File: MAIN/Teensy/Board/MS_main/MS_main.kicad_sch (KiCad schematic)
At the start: 32 parts, among them J1 External 5V, J10 RM_Motor, J11 RM_Motor, J12 Capacitive Soil Moisture Sens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, J14 LED, J15 LED_U, J16 RM_Motor, J17 RM_Motor, J18 RM_Motor, J19 RM_Motor, J2 BLD-510B_1, J20 RM_Motor, J21 Teensy4.1_Extention, J22 AE-PCA9685_Extention, J23 AE-PCA9685_Remaining, J3 BLD-510B_2, J4 BLD-510B_3, J5 BLD-510B_4, J6 BLD-510B_5, J7 SG_90-HV, J8 RM_Motor, J9 RM_Motor, U1 Teensy4.1

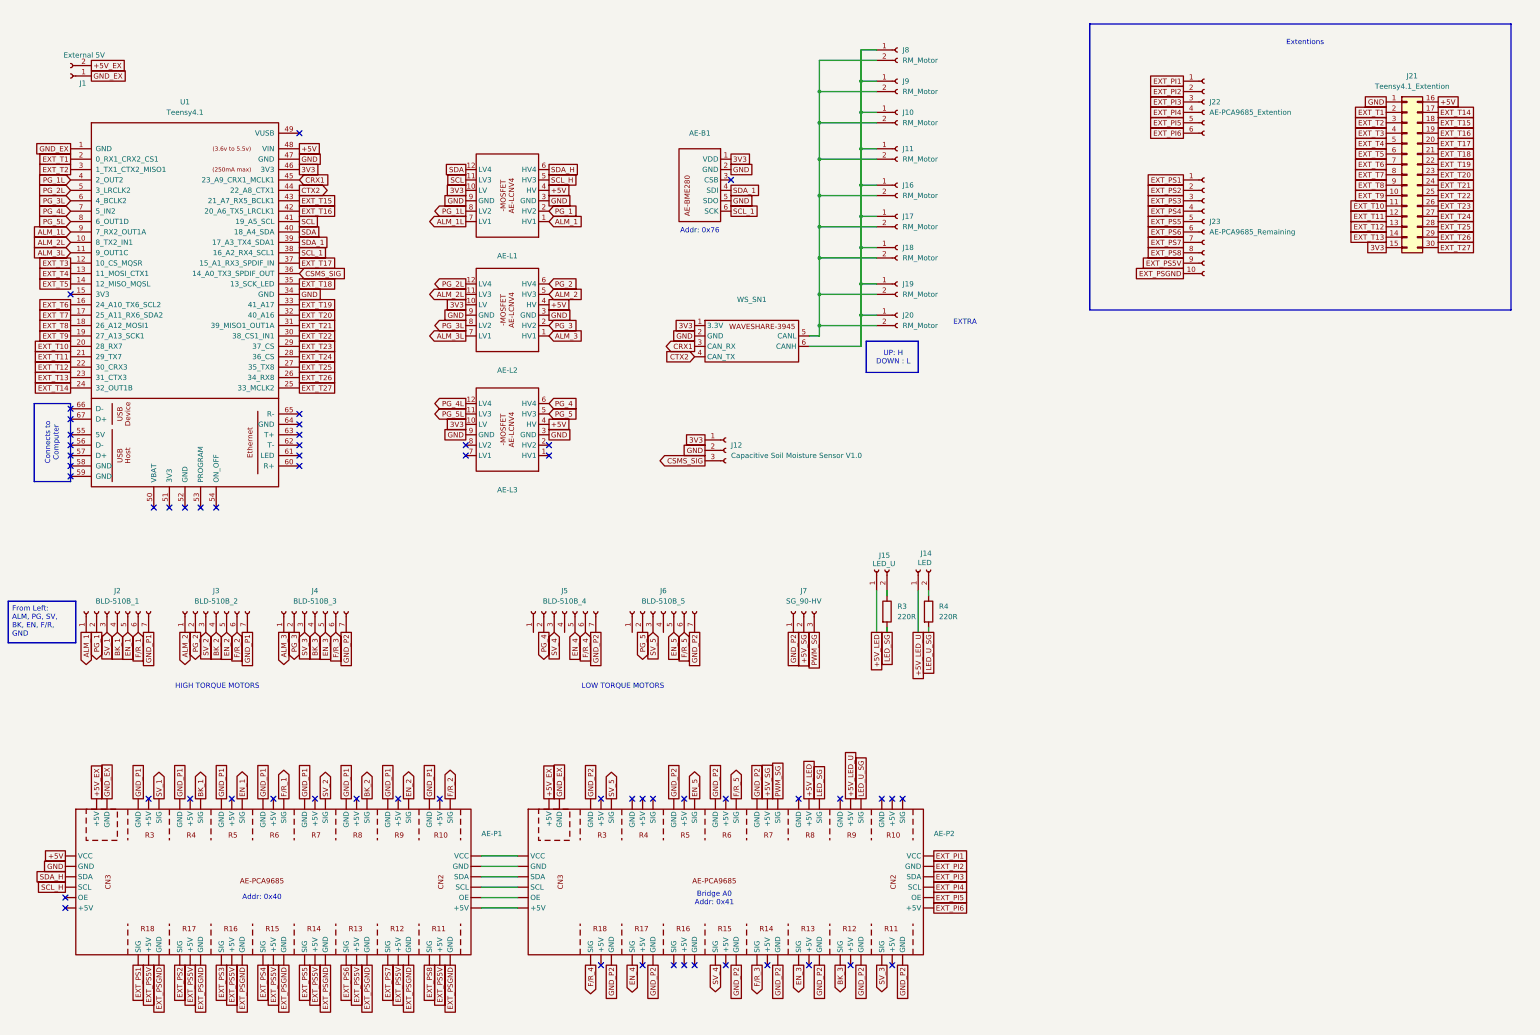
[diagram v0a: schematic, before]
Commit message: board revamp
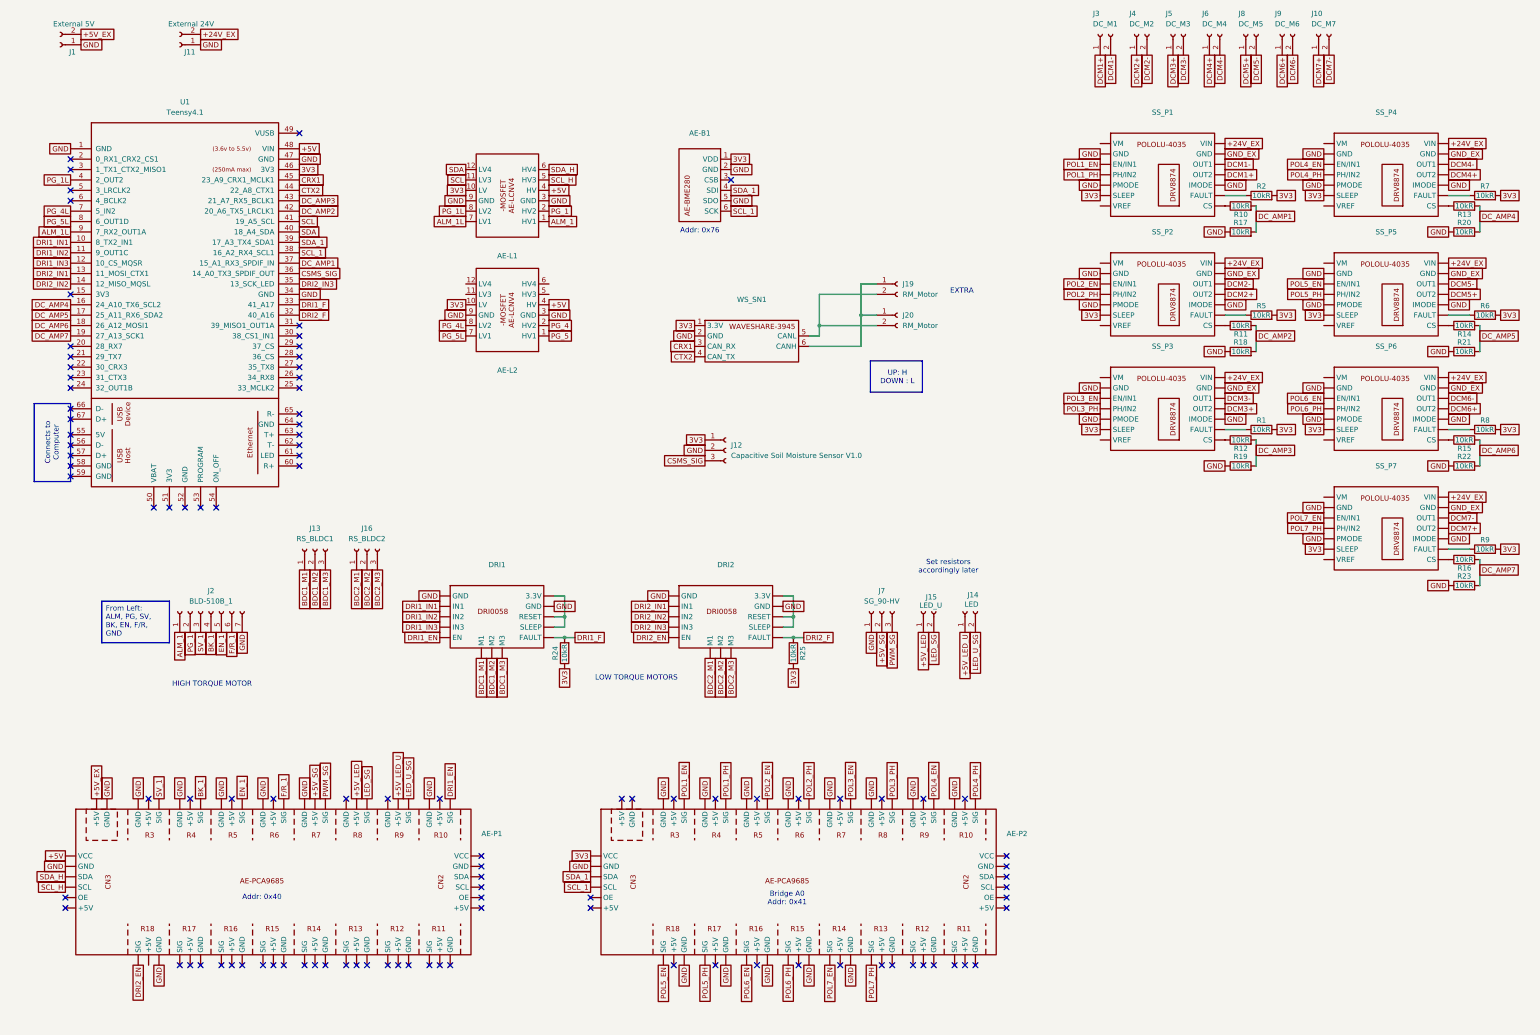
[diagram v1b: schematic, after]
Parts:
- removed AE-L3: ~, ALM_1L, symbol 1_MS_Parts:AE-LCNV4-MOSFET
- removed J16, J17, J18: RM_Motor, symbol Connector:Conn_01x02_Socket
- removed J21: Teensy4.1_Extention, symbol Connector_Generic:Conn_02x15_Top_Bottom
- removed J22: AE-PCA9685_Extention, symbol Connector:Conn_01x06_Socket
- removed J23: AE-PCA9685_Remaining, symbol Connector:Conn_01x10_Socket
- removed J3: BLD-510B_2, symbol Connector:Conn_01x07_Socket
- removed J4: BLD-510B_3, symbol Connector:Conn_01x07_Socket
- removed J5: BLD-510B_4, symbol Connector:Conn_01x07_Socket
- removed J6: BLD-510B_5, symbol Connector:Conn_01x07_Socket
- removed R3, R4: 220R, symbol Device:R
- added DRI1, DRI2: ~, symbol 1_MS_Parts:DRI0058
- added J13: RS_BLDC1, symbol Connector:Conn_01x03_Socket
- added J16: RS_BLDC2, symbol Connector:Conn_01x03_Socket
- added J3: DC_M1, symbol Connector:Conn_01x02_Socket
- added J4: DC_M2, symbol Connector:Conn_01x02_Socket
- added J5: DC_M3, symbol Connector:Conn_01x02_Socket
- added J6: DC_M4, symbol Connector:Conn_01x02_Socket
- added R1, R10, R11, R12, R13, R14, R15, R16, R17, R18, R19, R2, R20, R21, R22, R23, R24, R25, R5, R6, R7, R8, R9: 10kR, symbol Device:R
- added SS_P1, SS_P2, SS_P3, SS_P4, SS_P5, SS_P6, SS_P7: ~, symbol 1_MS_Parts:POLOLU-4035
- J10: value RM_Motor -> DC_M7
- J11: value RM_Motor -> External 24V
- J8: value RM_Motor -> DC_M5
- J9: value RM_Motor -> DC_M6
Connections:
- net ALM_3 is gone; now on net PG_5: AE-L2.1 (HV1)
- net BK_2 is gone; now on net SV_1: AE-P1. (VCC)
- net BK_3 is gone; now on net SDA_1: AE-P2. (VCC)
- net EN_2 is gone; now on net SV_1: AE-P1. (VCC)
- net EN_3 is gone; now on net SDA_1: AE-P2. (VCC)
- net EN_4 is gone; now on net SDA_1: AE-P2. (VCC)
- net EN_5 is gone; now on net SDA_1: AE-P2. (VCC)
- net EXT_PI1 is gone; now on net SDA_1: AE-P2. (VCC)
- net EXT_PI2 is gone; now on net SDA_1: AE-P2. (VCC)
- net EXT_PI3 is gone; now on net SDA_1: AE-P2. (VCC)
- net EXT_PI4 is gone; now on net SDA_1: AE-P2. (VCC)
- net EXT_PI5 is gone; now on net SDA_1: AE-P2. (VCC)
- net EXT_PI6 is gone; now on net SDA_1: AE-P2. (VCC)
- net EXT_PS1 is gone; now on net SV_1: AE-P1. (VCC)
- net EXT_PS2 is gone; now on net SV_1: AE-P1. (VCC)
- net EXT_PS3 is gone; now on net SV_1: AE-P1. (VCC)
- net EXT_PS4 is gone; now on net SV_1: AE-P1. (VCC)
- net EXT_PS5 is gone; now on net SV_1: AE-P1. (VCC)
- net EXT_PS5V is gone; now on net SV_1: AE-P1. (VCC)
- net EXT_PS6 is gone; now on net SV_1: AE-P1. (VCC)
- net EXT_PS7 is gone; now on net SV_1: AE-P1. (VCC)
- net EXT_PS8 is gone; now on net SV_1: AE-P1. (VCC)
- net EXT_PSGND is gone; now on net SV_1: AE-P1. (VCC)
- net F/R_2 is gone; now on net SV_1: AE-P1. (VCC)
- net F/R_3 is gone; now on net SDA_1: AE-P2. (VCC)
- net F/R_4 is gone; now on net SDA_1: AE-P2. (VCC)
- net F/R_5 is gone; now on net SDA_1: AE-P2. (VCC)
- net PG_3 is gone; now on net PG_4: AE-L2.2 (HV2)
- net SV_2 is gone; now on net SV_1: AE-P1. (VCC)
- net SV_3 is gone; now on net SDA_1: AE-P2. (VCC)
- net SV_4 is gone; now on net SDA_1: AE-P2. (VCC)
- net SV_5 is gone; now on net SDA_1: AE-P2. (VCC)
- net +5V_EX: no longer AE-P2. (VCC)
- net +5V_LED: now also AE-P1. (VCC); no longer AE-P2. (VCC)
- net +5V_LED_U: now also AE-P1. (VCC); no longer AE-P2. (VCC)
- net +5V_SG: now also AE-P1. (VCC); no longer AE-P2. (VCC)
- net 3V3: now also AE-P2. (VCC), R1.2, R2.2, R24.1, R25.2, R5.2, R6.2, R7.2, R8.2, R9.2, SS_P1. (CS), SS_P2. (CS), SS_P3. (CS), SS_P4. (CS), SS_P5. (CS), SS_P6. (CS), SS_P7. (CS)
- net GND: now also AE-P2. (VCC), J1.1 (Pin_1), J11.1 (Pin_1), J2.7 (Pin_7), J7.1 (Pin_1), U1.1 (GND), DRI1. (FAULT), DRI2. (FAULT), R17.1, R18.1, R19.1, R20.1, R21.1, R22.1, R23.1, SS_P1. (CS), SS_P2. (CS), SS_P3. (CS), SS_P4. (CS), SS_P5. (CS), SS_P6. (CS), SS_P7. (CS)
- net GND_EX: now also SS_P1. (CS), SS_P2. (CS), SS_P3. (CS), SS_P4. (CS), SS_P5. (CS), SS_P6. (CS), SS_P7. (CS); no longer AE-P1. (VCC), AE-P2. (VCC), J1.1 (Pin_1), U1.1 (GND)
- net LED_SG: now also AE-P1. (VCC), J15.2 (Pin_2); no longer AE-P2. (VCC)
- net LED_U_SG: now also AE-P1. (VCC), J14.2 (Pin_2); no longer AE-P2. (VCC)
- net PG_4L: now also AE-L2.8 (LV2)
- net PG_5L: now also AE-L2.7 (LV1)
- net PWM_SG: now also AE-P1. (VCC); no longer AE-P2. (VCC)
- net SCL_1: now also AE-P2. (VCC)
- net ALM_2: no longer names the net of AE-L2.5 (HV3)
- net ALM_2L: no longer names the net of AE-L2.11 (LV3)
- net ALM_2L: no longer U1.10 (8_TX2_IN1)
- net ALM_3L renamed DRI1_IN2
- net DRI1_IN2: now also DRI1. (FAULT); no longer AE-L2.7 (LV1)
- net EXT_T1: no longer names the net of U1.2 (0_RX1_CRX2_CS1)
- net EXT_T10: no longer names the net of U1.20 (28_RX7)
- net EXT_T11: no longer names the net of U1.21 (29_TX7)
- net EXT_T12: no longer names the net of U1.22 (30_CRX3)
- net EXT_T13: no longer names the net of U1.23 (31_CTX3)
- net EXT_T14: no longer names the net of U1.24 (32_OUT1B)
- net EXT_T15 renamed DC_AMP3
- net DC_AMP3: now also R12.2, R19.2
- net EXT_T16 renamed DC_AMP2
- net DC_AMP2: now also R11.2, R18.2
- net EXT_T17 renamed DC_AMP1
- net DC_AMP1: now also R10.2, R17.2
- net EXT_T18 renamed DRI2_IN3
- net DRI2_IN3: now also DRI2. (FAULT)
- net EXT_T19 renamed DRI1_F
- net DRI1_F: now also DRI1. (FAULT), R24.2
- net EXT_T2: no longer names the net of U1.3 (1_TX1_CTX2_MISO1)
- net EXT_T20 renamed DRI2_F
- net DRI2_F: now also DRI2. (FAULT), R25.1
- net EXT_T21: no longer names the net of U1.31 (39_MISO1_OUT1A)
- net EXT_T22: no longer names the net of U1.30 (38_CS1_IN1)
- net EXT_T23: no longer names the net of U1.29 (37_CS)
- net EXT_T24: no longer names the net of U1.28 (36_CS)
- net EXT_T25: no longer names the net of U1.27 (35_TX8)
- net EXT_T26: no longer names the net of U1.26 (34_RX8)
- net EXT_T27: no longer names the net of U1.25 (33_MCLK2)
- net EXT_T3 renamed DRI1_IN3
- net DRI1_IN3: now also DRI1. (FAULT)
- net EXT_T4 renamed DRI2_IN1
- net DRI2_IN1: now also DRI2. (FAULT)
- net EXT_T5 renamed DRI2_IN2
- net DRI2_IN2: now also DRI2. (FAULT)
- net EXT_T6 renamed DC_AMP4
- net DC_AMP4: now also R13.2, R20.2
- net EXT_T7 renamed DC_AMP5
- net DC_AMP5: now also R14.2, R21.2
- net EXT_T8 renamed DC_AMP6
- net DC_AMP6: now also R15.2, R22.2
- net EXT_T9 renamed DC_AMP7
- net DC_AMP7: now also R16.2, R23.2
- removed net GND_P1: AE-P1. (VCC), J2.7 (Pin_7)
- removed net GND_P2: AE-P2. (VCC), J7.1 (Pin_1)
- net PG_2: no longer names the net of AE-L2.6 (HV4)
- net PG_2L: no longer names the net of AE-L2.12 (LV4)
- net PG_2L: no longer U1.5 (3_LRCLK2)
- net PG_3L: no longer names the net of U1.6 (4_BCLK2)
- net PG_3L: no longer AE-L2.8 (LV2)
- new net: R11.1, SS_P2. (CS)
- new net: R13.1, SS_P4. (CS)
- new net: R1.1, SS_P3. (CS)
- new net: R5.1, SS_P2. (CS)
- new net: R8.1, SS_P6. (CS)
- new net: J19.1 (Pin_1), J20.1 (Pin_1), WS_SN1.6 (CANH)
- new net: J19.2 (Pin_2), J20.2 (Pin_2), WS_SN1.5 (CANL)
- new net: R2.1, SS_P1. (CS)
- new net: R14.1, SS_P5. (CS)
- new net: R7.1, SS_P4. (CS)
- new net: R9.1, SS_P7. (CS)
- new net: R12.1, SS_P3. (CS)
- new net: R15.1, SS_P6. (CS)
- new net: R10.1, SS_P1. (CS)
- new net: R16.1, SS_P7. (CS)
- new net: R6.1, SS_P5. (CS)
- new net +24V_EX: J11.2 (Pin_2), SS_P1. (CS), SS_P2. (CS), SS_P3. (CS), SS_P4. (CS), SS_P5. (CS), SS_P6. (CS), SS_P7. (CS)
- new net BDC1_M1: DRI1. (FAULT), J13.1 (Pin_1)
- new net BDC1_M2: DRI1. (FAULT), J13.2 (Pin_2)
- new net BDC1_M3: DRI1. (FAULT), J13.3 (Pin_3)
- new net BDC2_M1: DRI2. (FAULT), J16.1 (Pin_1)
- new net BDC2_M2: DRI2. (FAULT), J16.2 (Pin_2)
- new net BDC2_M3: DRI2. (FAULT), J16.3 (Pin_3)
- new net DCM1+: J3.1 (Pin_1), SS_P1. (CS)
- new net DCM1-: J3.2 (Pin_2), SS_P1. (CS)
- new net DCM2+: J4.1 (Pin_1), SS_P2. (CS)
- new net DCM2-: J4.2 (Pin_2), SS_P2. (CS)
- new net DCM3+: J5.1 (Pin_1), SS_P3. (CS)
- new net DCM3-: J5.2 (Pin_2), SS_P3. (CS)
- new net DCM4+: J6.1 (Pin_1), SS_P4. (CS)
- new net DCM4-: J6.2 (Pin_2), SS_P4. (CS)
- new net DCM5+: J8.1 (Pin_1), SS_P5. (CS)
- new net DCM5-: J8.2 (Pin_2), SS_P5. (CS)
- new net DCM6+: J9.1 (Pin_1), SS_P6. (CS)
- new net DCM6-: J9.2 (Pin_2), SS_P6. (CS)
- new net DCM7+: J10.1 (Pin_1), SS_P7. (CS)
- new net DCM7-: J10.2 (Pin_2), SS_P7. (CS)
- new net DRI1_EN: AE-P1. (VCC), DRI1. (FAULT)
- new net DRI1_IN1: DRI1. (FAULT), U1.10 (8_TX2_IN1)
- new net DRI2_EN: AE-P1. (VCC), DRI2. (FAULT)
- new net POL1_EN: AE-P2. (VCC), SS_P1. (CS)
- new net POL1_PH: AE-P2. (VCC), SS_P1. (CS)
- new net POL2_EN: AE-P2. (VCC), SS_P2. (CS)
- new net POL2_PH: AE-P2. (VCC), SS_P2. (CS)
- new net POL3_EN: AE-P2. (VCC), SS_P3. (CS)
- new net POL3_PH: AE-P2. (VCC), SS_P3. (CS)
- new net POL4_EN: AE-P2. (VCC), SS_P4. (CS)
- new net POL4_PH: AE-P2. (VCC), SS_P4. (CS)
- new net POL5_EN: AE-P2. (VCC), SS_P5. (CS)
- new net POL5_PH: AE-P2. (VCC), SS_P5. (CS)
- new net POL6_EN: AE-P2. (VCC), SS_P6. (CS)
- new net POL6_PH: AE-P2. (VCC), SS_P6. (CS)
- new net POL7_EN: AE-P2. (VCC), SS_P7. (CS)
- new net POL7_PH: AE-P2. (VCC), SS_P7. (CS)
- no-connect marks 56 -> 104
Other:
- note added: "HIGH TORQUE MOTOR"
- note added: "Set resistors accordingly later"
- note removed: "Extentions"
- note removed: "HIGH TORQUE MOTORS"
- moved on the sheet: AE-P2, J1, J14, J15, J2, J7

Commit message: update board
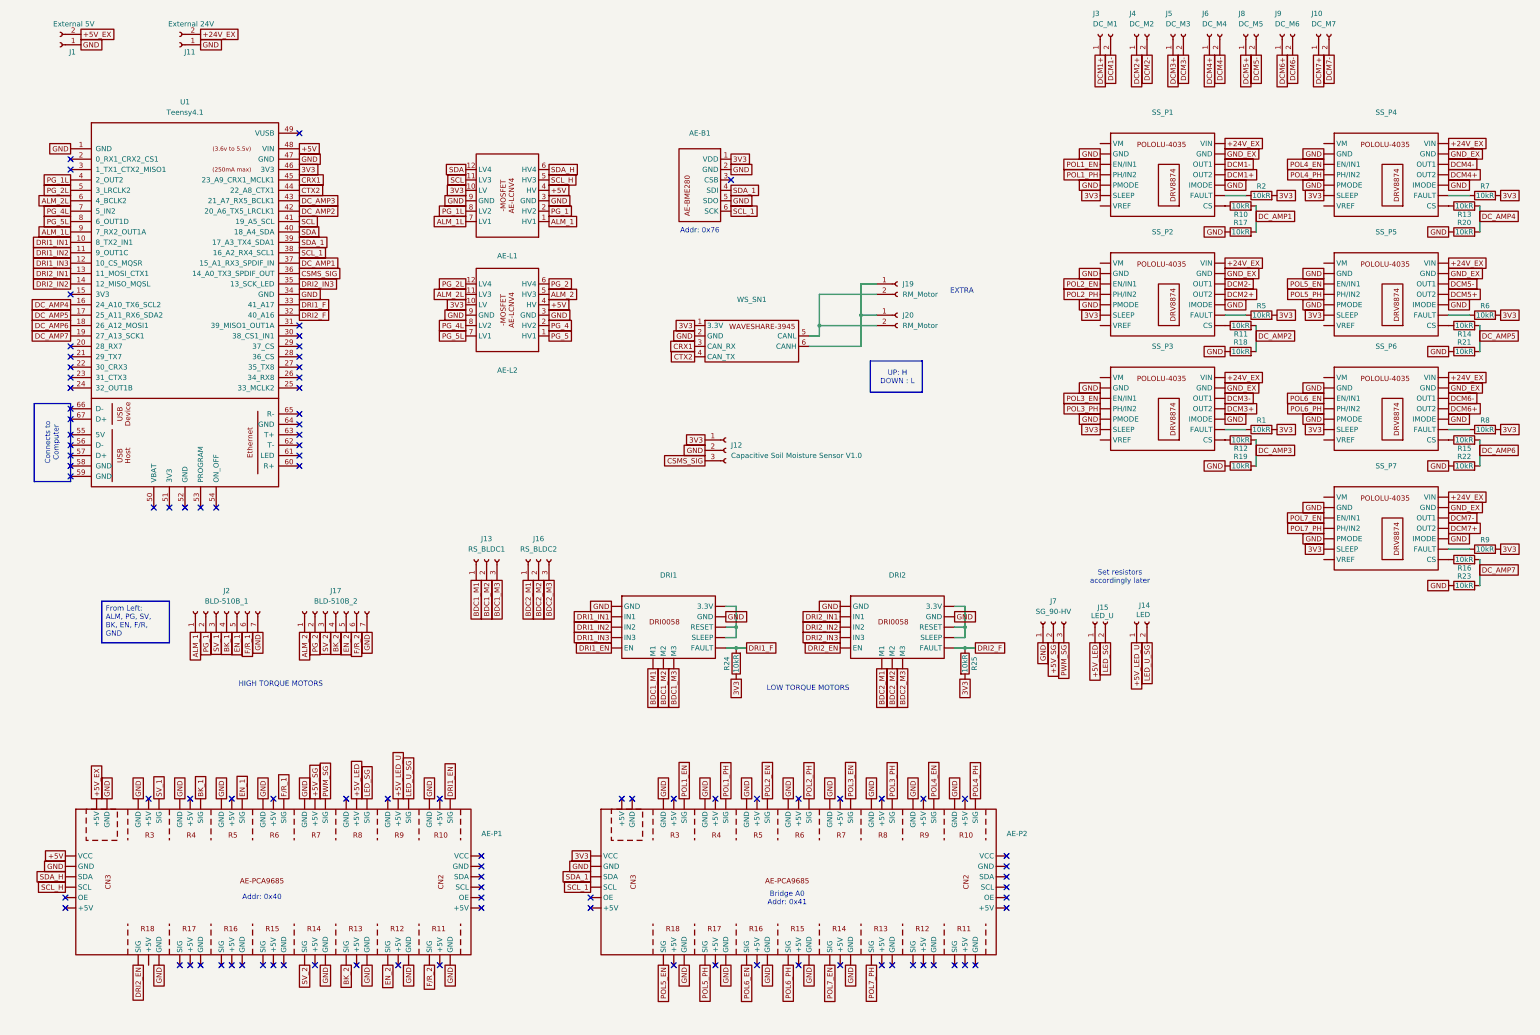
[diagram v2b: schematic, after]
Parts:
- added J17: BLD-510B_2, symbol Connector:Conn_01x07_Socket
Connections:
- net GND: now also J17.7 (Pin_7)
- net ALM_2L: now reaches AE-L2.11 (LV3)
- net ALM_2L: now also U1.6 (4_BCLK2)
- net PG_2L: now reaches AE-L2.12 (LV4)
- net PG_2L: now also U1.5 (3_LRCLK2)
- net ALM_2: now reaches AE-L2.5 (HV3)
- net ALM_2: now also J17.1 (Pin_1)
- net PG_2: now reaches AE-L2.6 (HV4)
- net PG_2: now also J17.2 (Pin_2)
- net SV_2: now reaches AE-P1. (VCC)
- net SV_2: now also J17.3 (Pin_3)
- new net BK_2: AE-P1. (VCC), J17.4 (Pin_4)
- new net EN_2: AE-P1. (VCC), J17.5 (Pin_5)
- new net F/R_2: AE-P1. (VCC), J17.6 (Pin_6)
- no-connect marks 104 -> 94
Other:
- note added: "HIGH TORQUE MOTORS"
- note removed: "HIGH TORQUE MOTOR"
- moved on the sheet: DRI1, DRI2, J13, J14, J15, J16, J2, J7, R24, R25
